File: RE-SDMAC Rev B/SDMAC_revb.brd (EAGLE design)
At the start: 100 x 80 mm, 13 parts, among them IC1 SUPER_DMAC_THT, U1 74ALVC164245DGGRE4DGG48-M, U3 74ALVC164245DGGRE4DGG48-M, U4 74ALVC164245DGGRE4DGG48-M, U5 74ALVC164245DGGRE4DGG48-M

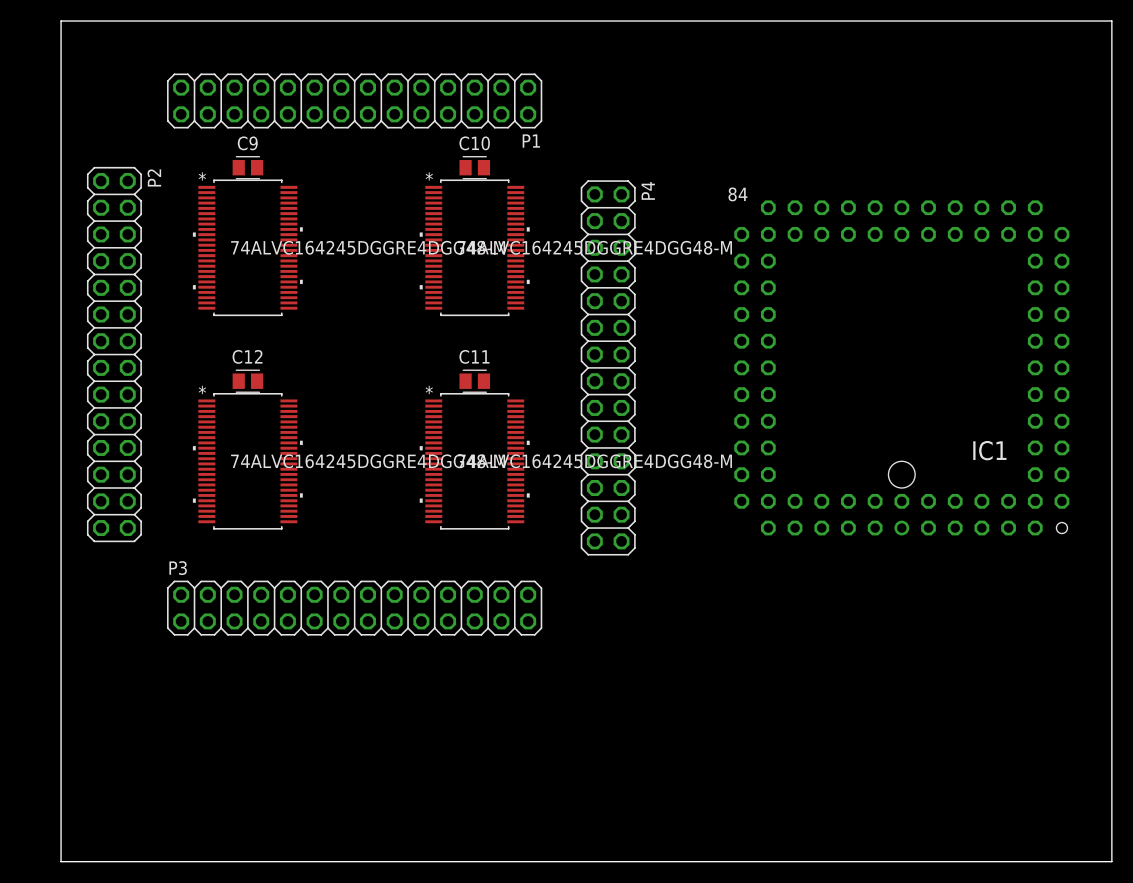
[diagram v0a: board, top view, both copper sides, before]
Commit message: quatus and rev b update
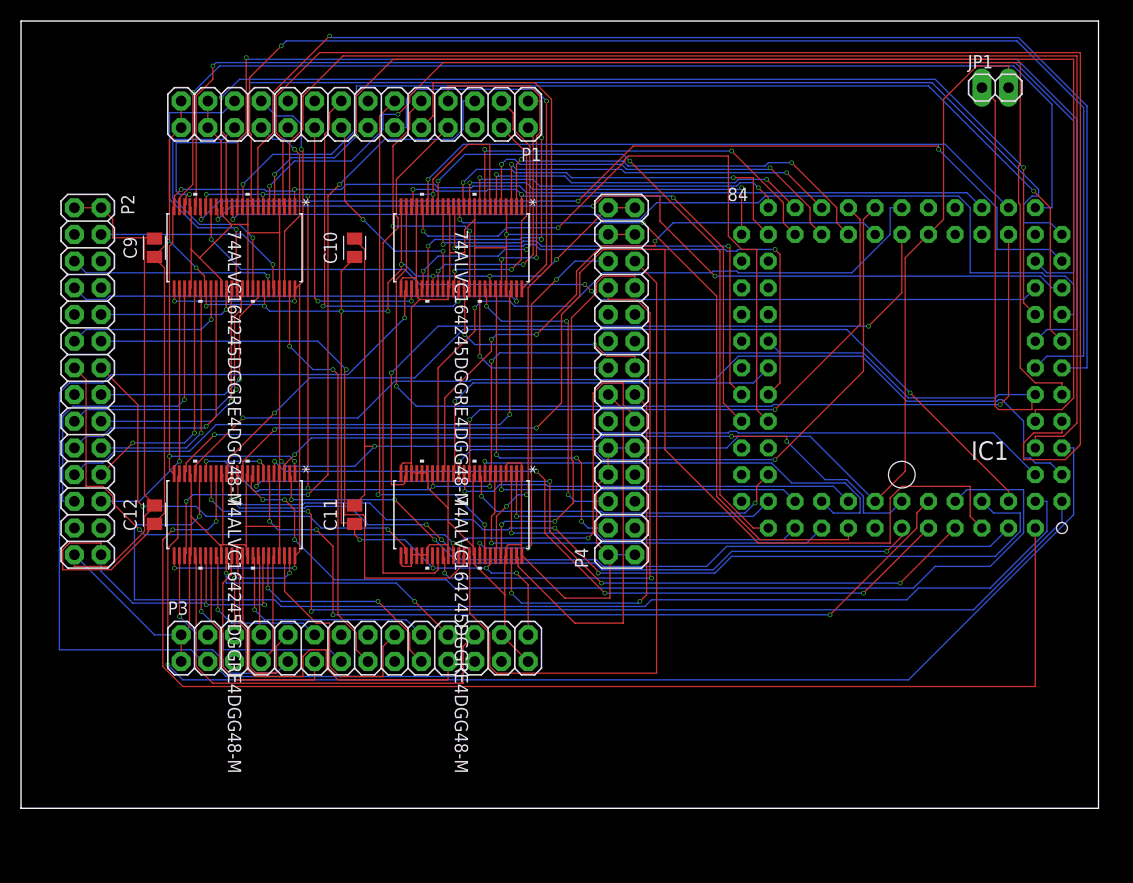
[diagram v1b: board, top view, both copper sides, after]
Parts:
- added JP1: (no value), pinhead:1X02
- moved U1 34.2 mm to (16.5, 33.0), turned to 270 degrees
- moved U5 32.5 mm to (38.1, 33.0), turned to 270 degrees
- moved U3 30.6 mm to (16.5, 58.4), turned to 270 degrees
- moved U4 28.7 mm to (38.1, 58.4), turned to 270 degrees
- moved C11 17.1 mm to (27.9, 33.0), turned to 90 degrees
- moved C12 15.5 mm to (8.89, 33.0), turned to 90 degrees
- moved C10 13.7 mm to (27.9, 58.4), turned to 90 degrees
- moved C9 11.7 mm to (8.89, 58.4), turned to 90 degrees
- moved P3 3.81 mm to (27.9, 20.3)
- moved P2 3.59 mm to (2.54, 45.7)
- moved P4 1.80 mm to (53.3, 45.7), turned to 90 degrees
- moved P1 1.27 mm to (27.9, 71.1)
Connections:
- removed net P1-1: U4.30
- new net P1_HDR1: P1.1, U4.30
- new net P1_HDR10: P1.10, U5.43
- new net P1_HDR11: P1.11, U5.41
- new net P1_HDR12: P1.12, U4.48
- new net P1_HDR13: P1.13
- new net P1_HDR14: P1.14
- new net P1_HDR15: P1.15, U4.36
- new net P1_HDR16: P1.16, U4.33
- new net P1_HDR17: P1.17
- new net P1_HDR18: P1.18, U4.27
- new net P1_HDR19: P1.19
- new net P1_HDR2: P1.2, U4.32
- new net P1_HDR20: P1.20
- new net P1_HDR22: P1.22, U3.46
- new net P1_HDR23: P1.23, U3.37
- new net P1_HDR24: P1.24, U3.40
- new net P1_HDR3: P1.3, U4.29
- new net P1_HDR4: P1.4, U4.35
- new net P1_HDR5: P1.5, U1.27
- new net P1_HDR6: P1.6
- new net P1_HDR7: P1.7, U4.44
- new net P1_HDR8: P1.8, U5.32
- new net P1_HDR9: P1.9, U4.38
- new net P2_HDR10: P2.10, U3.35
- new net P2_HDR11: P2.11, U3.32
- new net P2_HDR12: P2.12, U5.37
- new net P2_HDR13: P2.13, U5.35
- new net P2_HDR14: P2.14, U5.26
- new net P2_HDR15: P2.15
- new net P2_HDR16: P2.16, U3.41
- new net P2_HDR17: P2.17, U3.38
- new net P2_HDR18: P2.18, U3.36
- new net P2_HDR19: P2.19, U3.33
- new net P2_HDR20: P2.20, U3.30
- new net P2_HDR21: P2.21, U4.46
- new net P2_HDR22: P2.22, U3.29
- new net P2_HDR23: P2.23, U3.27
- new net P2_HDR24: P2.24, U3.26
- new net P2_HDR25: P2.25
- new net P2_HDR26: P2.26
- new net P2_HDR3: P2.3
- new net P2_HDR4: P2.4, U3.44
- new net P2_HDR5: P2.5, U3.43
- new net P2_HDR6: P2.6
- new net P2_HDR7: P2.7, U4.47
- new net P2_HDR8: P2.8
- new net P2_HDR9: P2.9
- new net P3_HDR10: P3.10, U1.38
- new net P3_HDR11: P3.11, U1.36
- new net P3_HDR12: P3.12, U1.33
- new net P3_HDR13: P3.13, U1.30
- new net P3_HDR14: P3.14
- new net P3_HDR15: P3.15, U3.47
- new net P3_HDR16: P3.16
- new net P3_HDR17: P3.17
- new net P3_HDR18: P3.18, U1.46
- new net P3_HDR19: P3.19, U1.43
- new net P3_HDR20: P3.20, U1.40
- new net P3_HDR21: P3.21, U1.37
- new net P3_HDR22: P3.22, U1.35
- new net P3_HDR23: P3.23, U1.32
- new net P3_HDR24: P3.24, U1.29
- new net P3_HDR25: P3.25
- new net P3_HDR3: P3.3, U4.26
- new net P3_HDR4: P3.4
- new net P3_HDR5: P3.5
- new net P3_HDR6: P3.6, U1.47
- new net P3_HDR7: P3.7, U1.44
- new net P3_HDR8: P3.8, U1.41
- new net P3_HDR9: P3.9, U1.26
- new net P4_HDR11: P4.11, U5.36
- new net P4_HDR12: P4.12
- new net P4_HDR13: P4.13, U5.46
- new net P4_HDR14: P4.14, U5.47
- new net P4_HDR15: P4.15, U4.37
- new net P4_HDR16: P4.16, U4.40
- new net P4_HDR17: P4.17
- new net P4_HDR18: P4.18
- new net P4_HDR21: P4.21, U5.44
- new net P4_HDR22: P4.22, U5.33
- new net P4_HDR23: P4.23, U5.38
- new net P4_HDR24: P4.24, U5.40
- new net P4_HDR3: P4.3
- new net P4_HDR4: P4.4, U4.43
- new net P4_HDR5: P4.5
- new net P4_HDR6: P4.6, U4.41
- new net P4_HDR7: P4.7
- net !CSS: no longer U4.48
- net !DATAOE: now also P1.21
- net GND: now also JP1.2, P1.25, P1.26, P2.1, P2.2, P2.27, P3.1, P3.2, P3.26, P3.27, P4.1, P4.10, P4.2, P4.25, P4.26, P4.8, P4.9, U5.27, U5.29, U5.30
- net VCC3.3: now also P1.27, P1.28, P2.28, P3.28, P4.27, P4.28
- net VCC5: now also JP1.1
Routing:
- net GND: track 0.00 -> 487.1 mm, vias 0 -> 3
- net VCC3.3: track 0.00 -> 207.2 mm, vias 0 -> 16
- net VCC5: track 0.00 -> 206.4 mm, vias 0 -> 10
- net CPU_DATAD17: track 0.00 -> 139.1 mm
- net CPU_DATAD16: track 0.00 -> 126.8 mm
- net CPU_DATAD21: track 0.00 -> 124.6 mm, vias 0 -> 1
- net CPU_DATAD18: track 0.00 -> 123.4 mm, vias 0 -> 2
- net CPU_DATAD10: track 0.00 -> 121.3 mm, vias 0 -> 2
- net CPU_DATAD20: track 0.00 -> 121.2 mm, vias 0 -> 1
- net CPU_DATAD23: track 0.00 -> 120.5 mm, vias 0 -> 1
- net R!W: track 0.00 -> 120.3 mm, vias 0 -> 4
- net CPU_DATAD15: track 0.00 -> 119.4 mm, vias 0 -> 1
- net CPU_DATAD29: track 0.00 -> 117.0 mm, vias 0 -> 1
- net CPU_DATAD6: track 0.00 -> 116.9 mm, vias 0 -> 2
- net CPU_DATAD19: track 0.00 -> 114.4 mm, vias 0 -> 2
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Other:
- board size 100 x 80 mm -> 102.5 x 74.9 mm
